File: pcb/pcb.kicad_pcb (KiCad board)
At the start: 2 copper layers, 64 parts, among them J1 WH, J2 RGB, J3 220, Q1 AO3400A, Q2 AO3400A, Q3 AO3400A, Q4 AO3400A, Q5 AOD452, Q6 DTD114E, Q7 AO3400A, SW1 mode, SW2 bright, T1 ., U1 ATtiny13A-SS, U2 TNY268G, U3 PC817, U4 TL431DBZ, U5 AZ1117-5.0

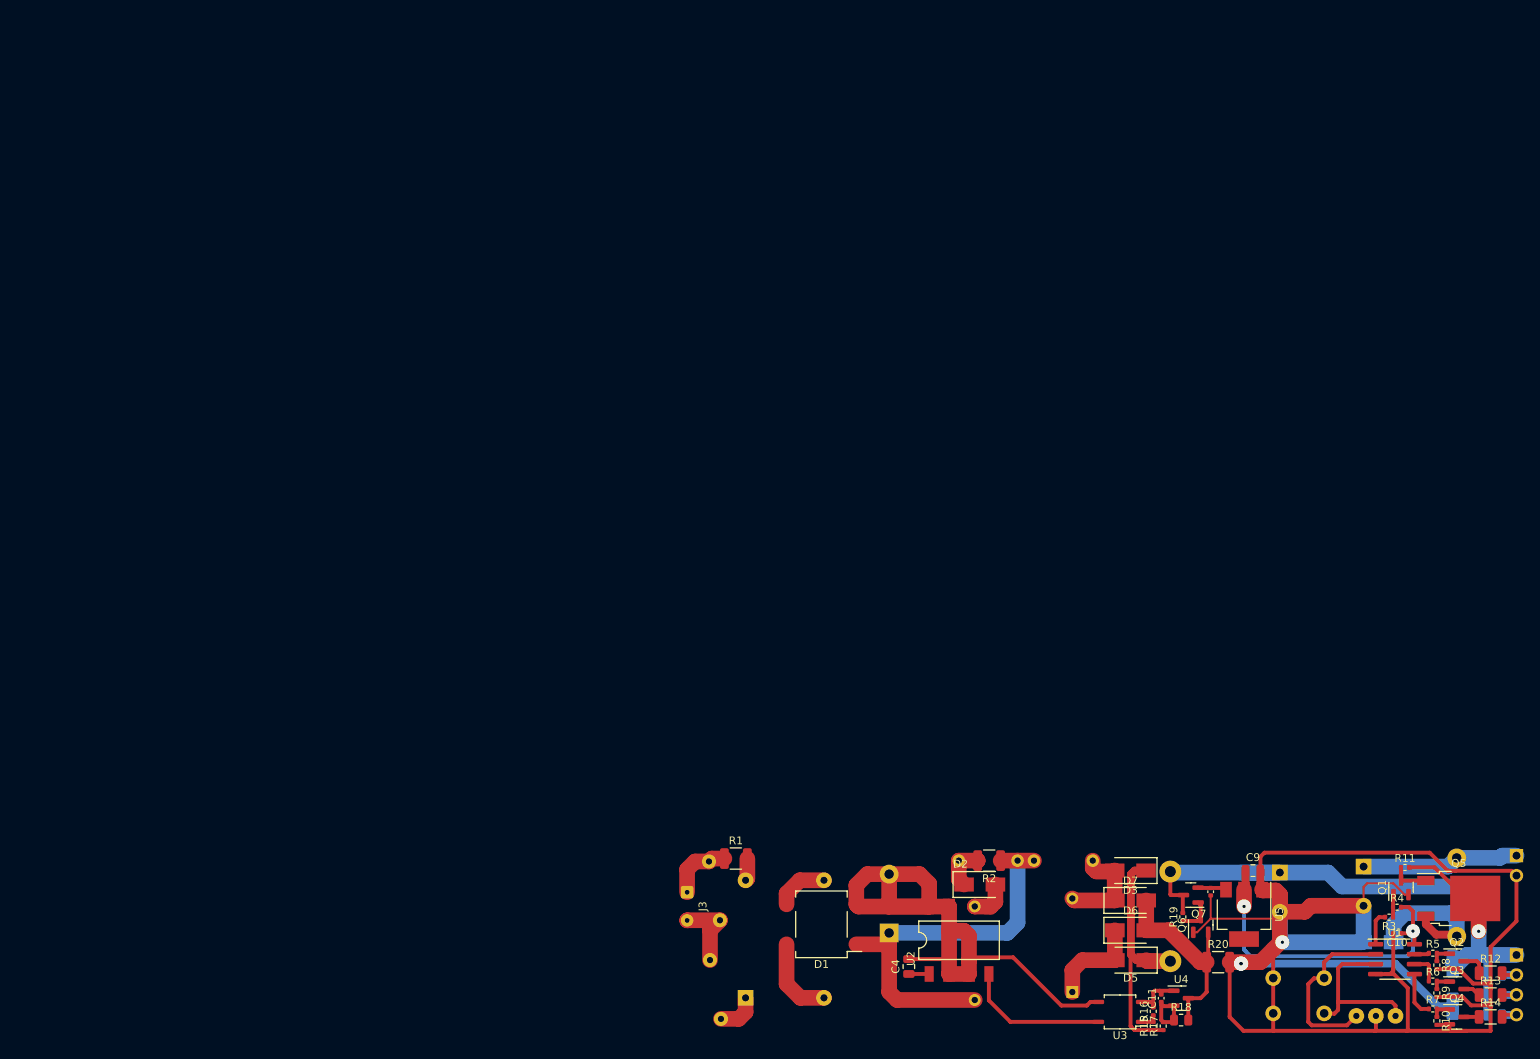
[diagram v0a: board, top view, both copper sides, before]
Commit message: operate led
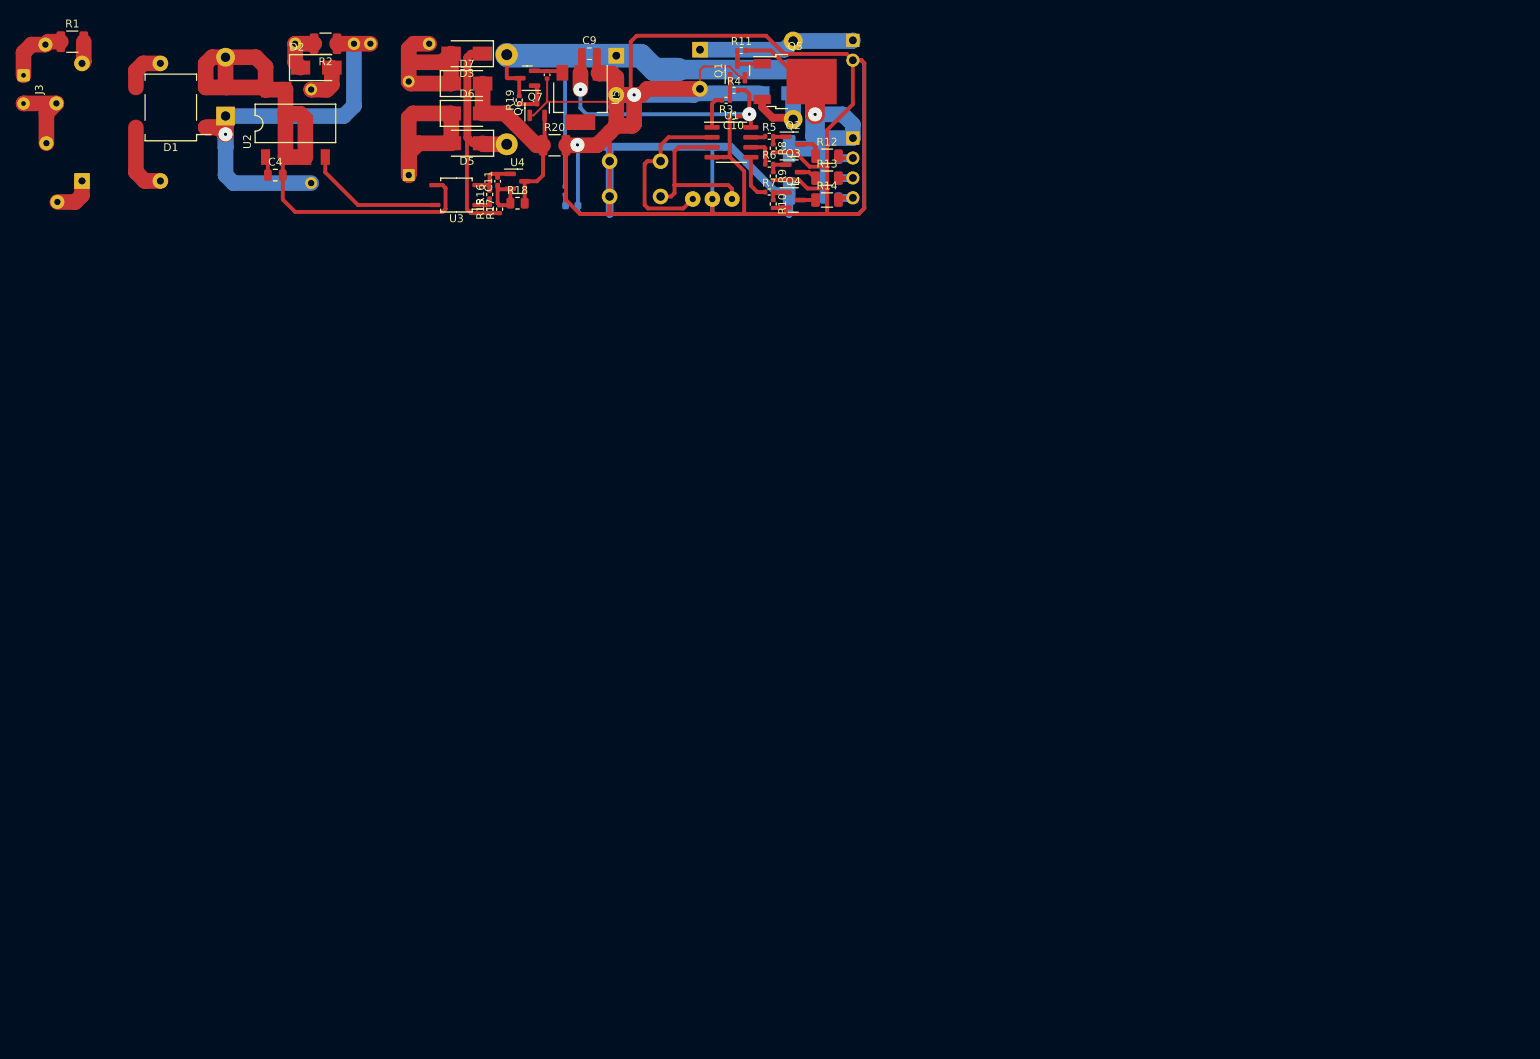
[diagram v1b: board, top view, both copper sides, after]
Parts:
- added D8: LED, LED_SMD:LED_0603_1608Metric, B.Cu at (109.0, 49.3)
- added R21: 1k, Resistor_SMD:R_0402_1005Metric, B.Cu at (108.1, 47.4)
- moved C1 134.3 mm to (64.8, 37.8)
- moved C10 134.3 mm to (129.6, 37.9)
- moved C3 134.3 mm to (83.3, 28.6)
- moved C5 134.3 mm to (125.3, 29.4)
- moved C7 134.3 mm to (114.7, 30.1)
- moved J2 134.3 mm to (144.9, 40.7)
- moved L2 134.3 mm to (137.2, 38.3)
- moved L3 134.3 mm to (100.7, 41.5)
- moved Q1 134.3 mm to (130.1, 32.0)
- moved Q2 134.3 mm to (137.2, 41.5)
- moved Q4 134.3 mm to (137.2, 48.6)
- moved R19 134.3 mm to (102.3, 35.8)
- moved R6 134.3 mm to (134.2, 44.0)
- moved R8 134.3 mm to (134.7, 42.0)
- moved RV1 134.3 mm to (43.2, 36.2)
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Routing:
- net GND: track 251.0 -> 369.6 mm, vias 3 -> 2
- net +12V: track 92.9 -> 113.9 mm
- net Net-(D5-Pad2): track 12.6 -> 25.5 mm
- net Net-(D4-Pad1): track 18.7 -> 8.96 mm
- net Net-(C3-Pad2): track 13.2 -> 22.4 mm
- net +5V: track 43.5 -> 36.9 mm
- net Net-(C1-Pad1): track 53.5 -> 58.8 mm, vias 0 -> 1
- net Net-(D8-Pad2): track 0.00 -> 1.43 mm
- net Net-(D1-Pad4): track 10.6 -> 9.29 mm
- net Net-(D1-Pad3): track 6.85 -> 5.65 mm
- net Net-(C1-Pad2): track 80.3 -> 79.4 mm
- net Net-(U2-Pad4): track 18.5 -> 17.7 mm

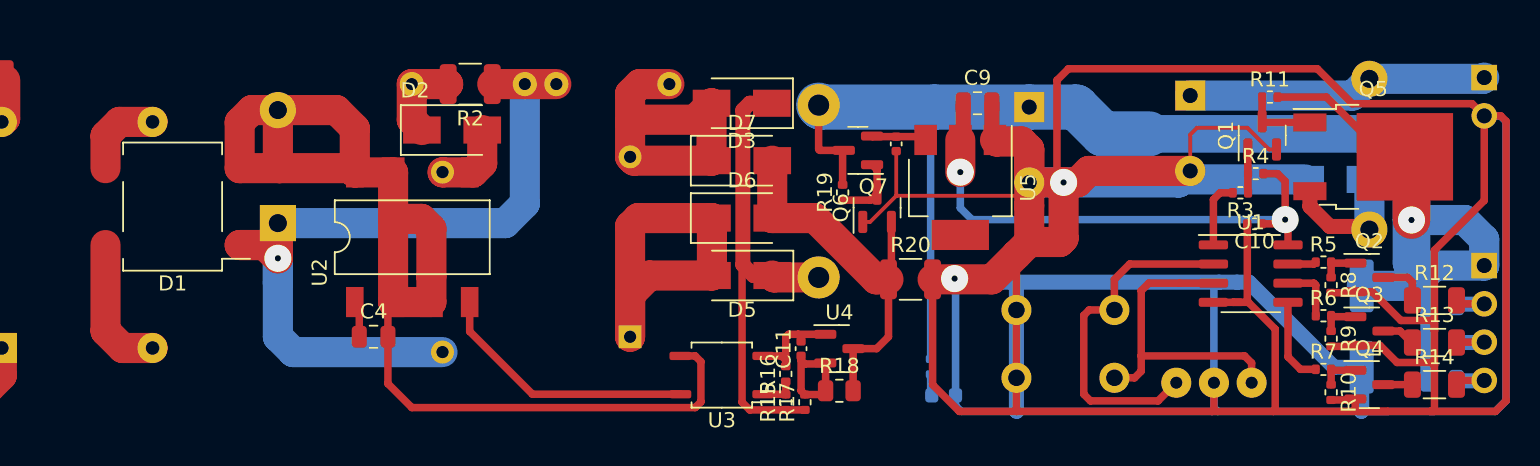
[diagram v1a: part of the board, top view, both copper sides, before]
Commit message: -2cm
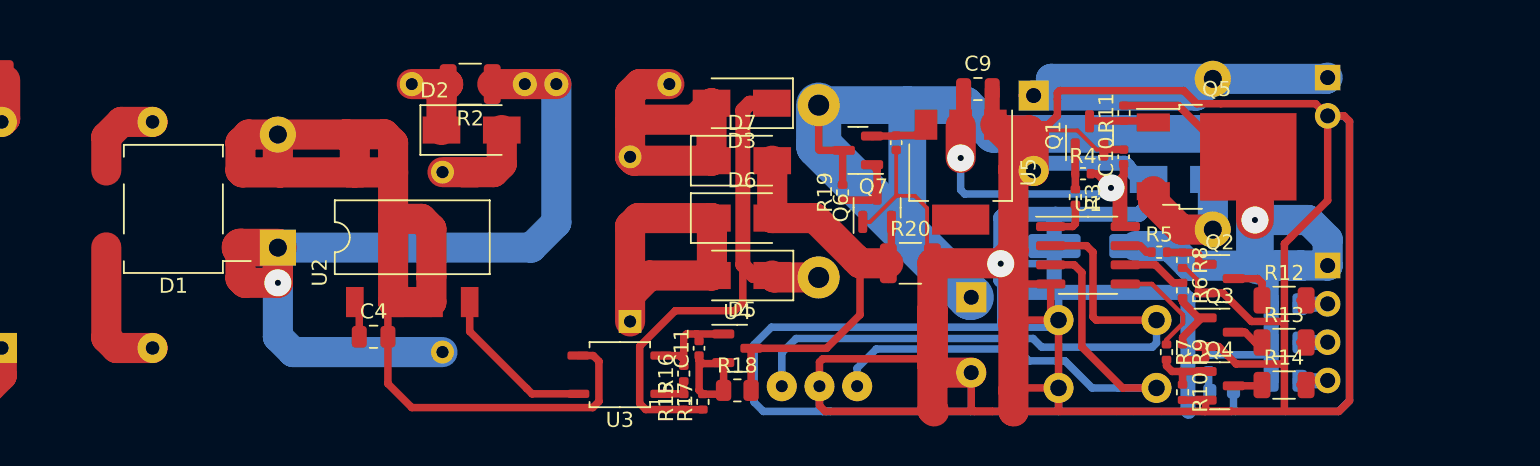
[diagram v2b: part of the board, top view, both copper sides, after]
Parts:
- moved SW2 26.2 mm to (100.8, 48.7)
- moved C6 18.5 mm to (119.0, 39.4), turned to 180 degrees
- moved D8 18.4 mm to (127.4, 49.0)
- moved R21 18.4 mm to (126.6, 47.1)
- moved C7 13.2 mm to (110.8, 42.8)
- moved R4 11.5 mm to (118.2, 34.6)
- moved Q1 11.5 mm to (118.7, 32.0)
- moved R3 11.0 mm to (117.7, 36.1), turned to -90 degrees
- moved R5 10.9 mm to (123.3, 39.8)
- moved U1 10.9 mm to (118.6, 40.0)
- moved R7 10.5 mm to (123.8, 46.4), turned to -90 degrees
- moved C12 10.4 mm to (131.7, 45.8)
- moved C13 10.4 mm to (131.7, 48.3)
- moved C14 10.4 mm to (131.7, 43.2)
- moved J1 10.4 mm to (134.5, 28.2)
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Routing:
- net Net-(SW1-Pad3): track 23.6 -> 40.9 mm
- net GND: track 369.6 -> 386.1 mm, vias 2 -> 1
- net Net-(SW1-Pad1): track 21.1 -> 36.0 mm
- net Net-(C5-Pad1): track 20.0 -> 30.8 mm
- net +5V: track 36.9 -> 28.1 mm
- net +12V: track 113.9 -> 122.1 mm
- net Net-(U2-Pad4): track 17.7 -> 10.9 mm
- net Net-(C1-Pad2): track 79.4 -> 73.9 mm
- net Net-(D3-Pad1): track 31.9 -> 37.0 mm
- net Net-(D6-Pad2): track 26.4 -> 31.0 mm
- net Net-(D5-Pad2): track 25.5 -> 21.7 mm
- net Net-(Q3-Pad1): track 2.64 -> 4.75 mm
- net Net-(R3-Pad2): track 4.40 -> 2.98 mm
- net Net-(Q4-Pad1): track 2.64 -> 4.05 mm
- net Net-(D2-Pad2): track 5.10 -> 6.40 mm
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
